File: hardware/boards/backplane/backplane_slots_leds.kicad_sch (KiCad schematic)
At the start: 19 parts, among them J1 DC_IN_SCREW_TERMINAL, J10 I2C_CHAIN_IN, J11 I2C_CHAIN_OUT, J12 LED_EXT_OUT, J14 LED_EXT_IN, J2 XT30U(2+2)-F.G.B_SLOT1, J3 XT30U(2+2)-F.G.B_SLOT2, J4 XT30U(2+2)-F.G.B_SLOT3, J5 XT30U(2+2)-F.G.B_SLOT4, J6 XT30U(2+2)-F.G.B_SLOT5, J7 XT30U(2+2)-F.G.B_SLOT6, J8 LED_EXT_IN, J9 DC_CHAIN_OUT

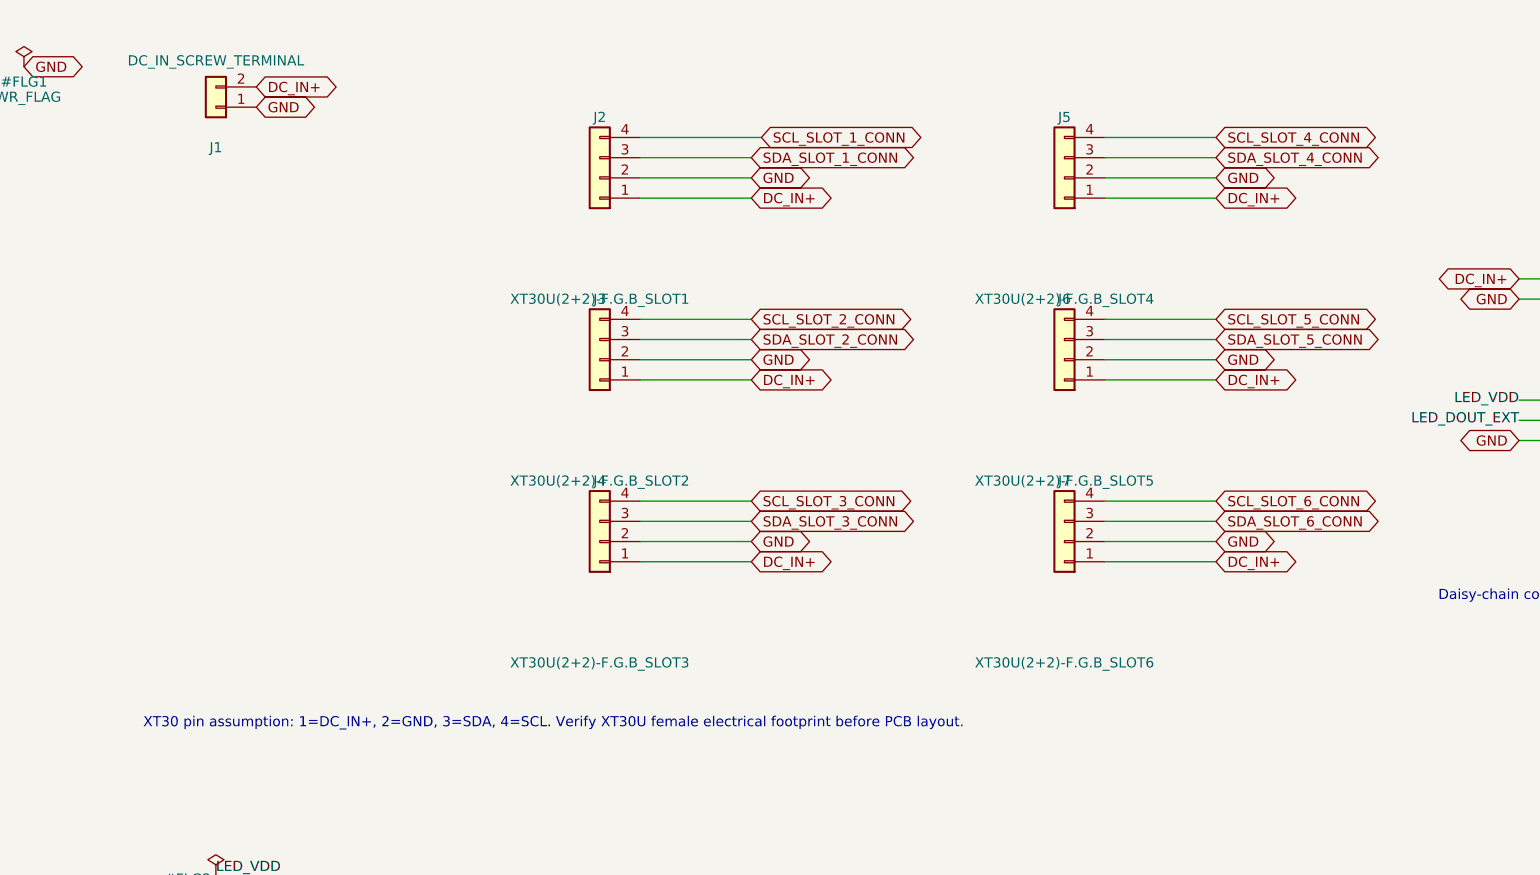
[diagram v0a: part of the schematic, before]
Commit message: Starrting to move things around
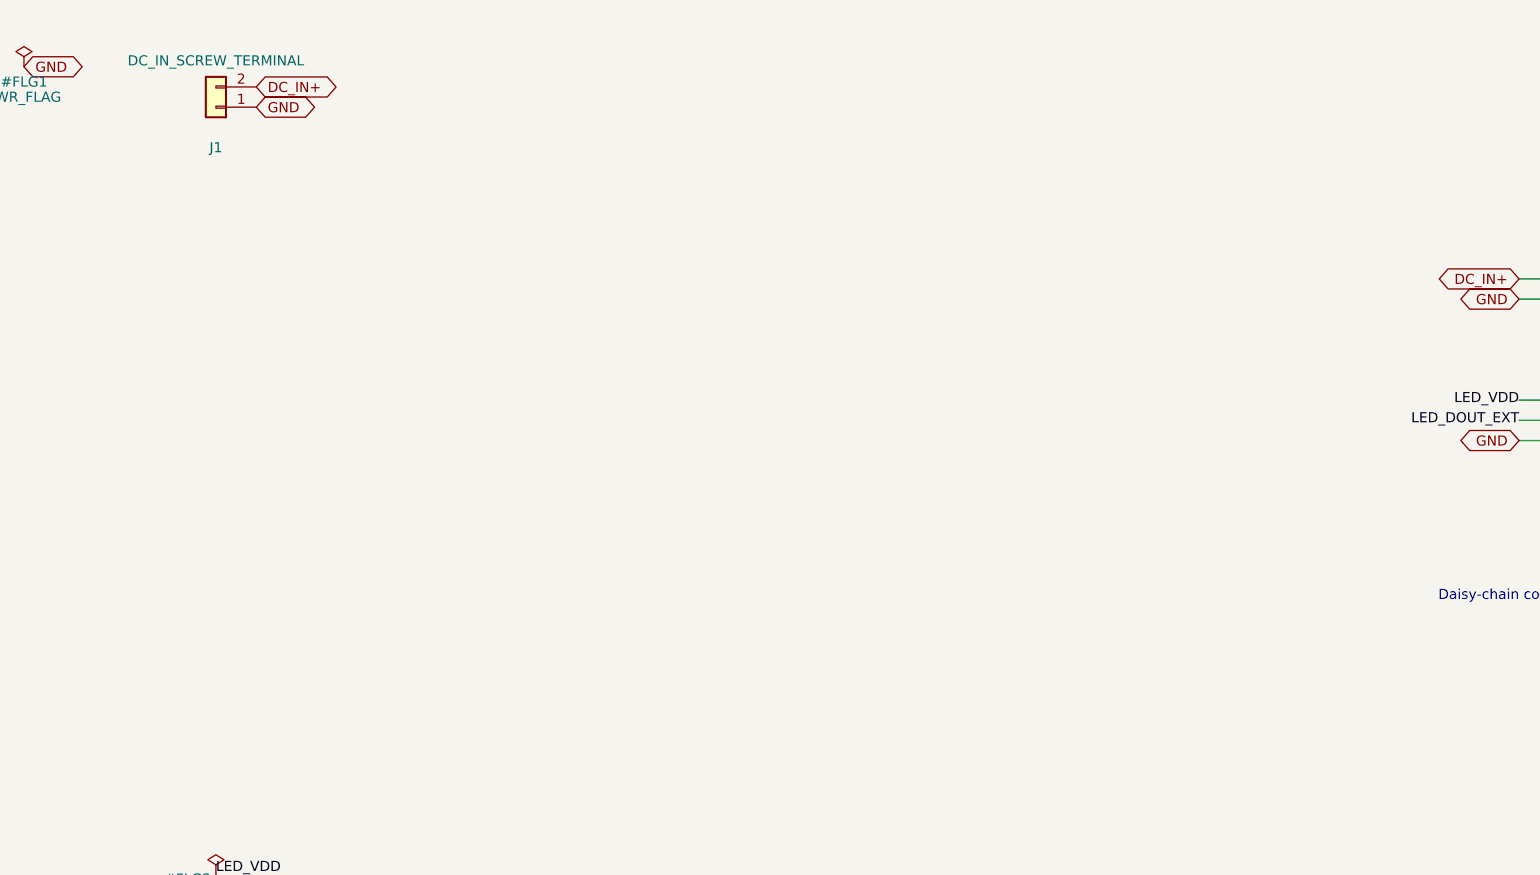
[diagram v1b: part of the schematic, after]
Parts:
- removed J2: XT30U(2+2)-F.G.B_SLOT1, mini-rack-power:Amass_XT30U_2plus2_F, symbol Connector_Generic:Conn_01x04
- removed J3: XT30U(2+2)-F.G.B_SLOT2, mini-rack-power:Amass_XT30U_2plus2_F, symbol Connector_Generic:Conn_01x04
- removed J4: XT30U(2+2)-F.G.B_SLOT3, mini-rack-power:Amass_XT30U_2plus2_F, symbol Connector_Generic:Conn_01x04
- removed J5: XT30U(2+2)-F.G.B_SLOT4, mini-rack-power:Amass_XT30U_2plus2_F, symbol Connector_Generic:Conn_01x04
- removed J6: XT30U(2+2)-F.G.B_SLOT5, mini-rack-power:Amass_XT30U_2plus2_F, symbol Connector_Generic:Conn_01x04
- removed J7: XT30U(2+2)-F.G.B_SLOT6, mini-rack-power:Amass_XT30U_2plus2_F, symbol Connector_Generic:Conn_01x04
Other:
- note removed: "XT30 pin assumption: 1=DC_IN+, 2=GND, 3=SDA, 4=SCL. Verify XT30U female electrical footprint before PCB layout."
